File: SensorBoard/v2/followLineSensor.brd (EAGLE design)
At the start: 102.5 x 34.3 mm, 24 parts

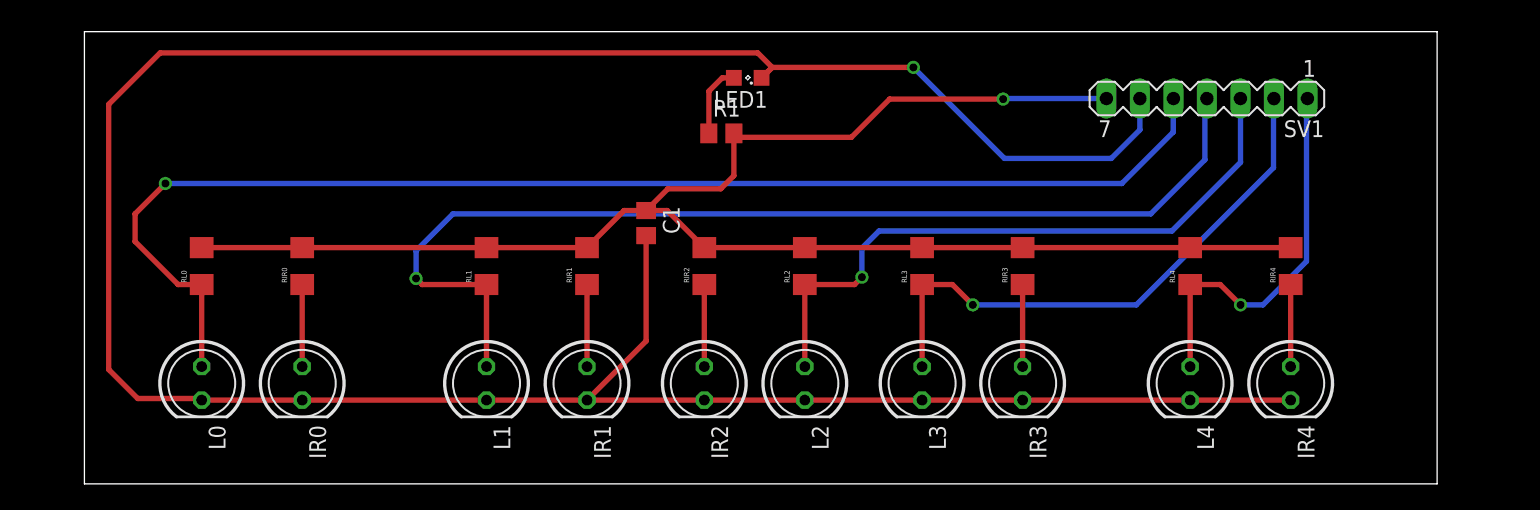
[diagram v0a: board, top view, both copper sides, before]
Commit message: Another better versions of the boards done
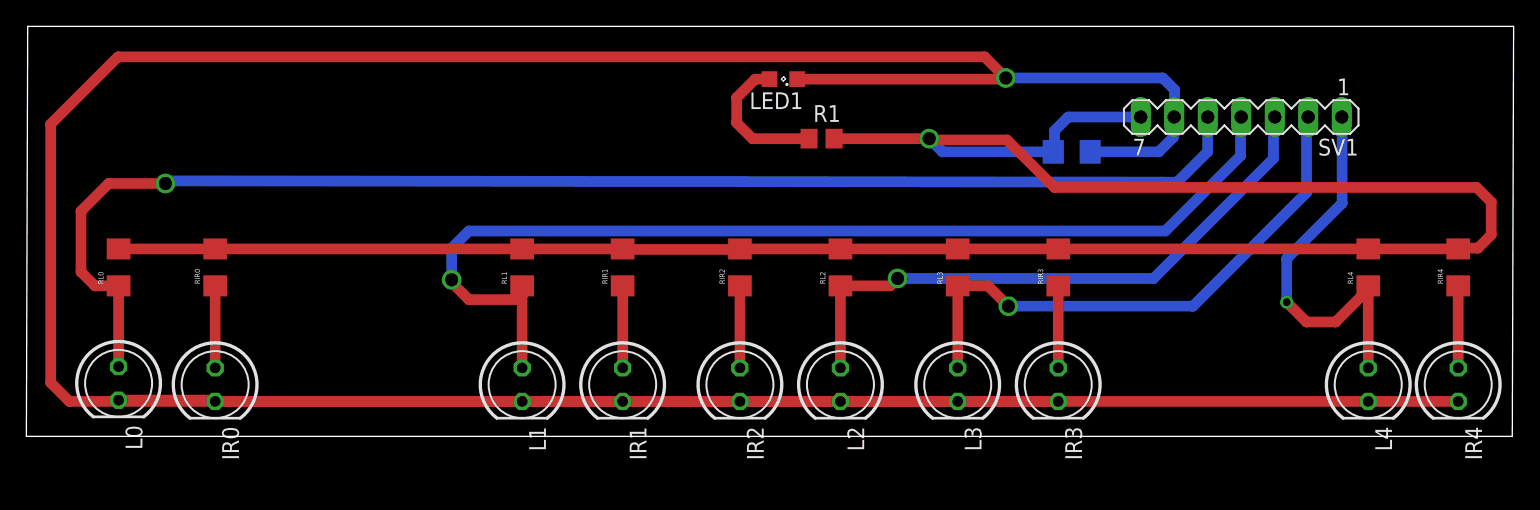
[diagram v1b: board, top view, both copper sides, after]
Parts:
- removed C1: 100nF, rcl:C0805
- added C2: 1uF, rcl:C1206
- moved L4 13.5 mm to (94.8, 44.4)
- moved RL4 13.5 mm to (94.8, 53.2)
- moved IR4 12.7 mm to (101.6, 44.4)
- moved RIR4 12.7 mm to (101.6, 53.2)
- moved R1 7.61 mm to (53.3, 63.0)
- moved IR0 6.60 mm to (7.37, 44.4)
- moved RIR0 6.60 mm to (7.37, 53.2)
- moved RL0 6.30 mm to (0.05, 53.2)
- moved L0 6.30 mm to (0.05, 44.5)
- moved SV1 2.95 mm to (85.2, 64.6)
- moved IR3 2.70 mm to (71.3, 44.4)
- moved L2 2.70 mm to (54.8, 44.4)
- moved RIR3 2.70 mm to (71.3, 53.2)
- moved RL2 2.70 mm to (54.8, 53.2)
- moved L1 2.70 mm to (30.6, 44.4)
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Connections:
- net GND: now also C2.2; no longer C1.2
- net VBAT: now also C2.1; no longer C1.1
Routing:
- net GND: track 213.6 -> 312.8 mm
- net VBAT: track 125.4 -> 177.3 mm
- net N$2: track 5.51 -> 11.0 mm
- net A0: track 98.5 -> 104.0 mm
- net A2: track 49.2 -> 46.4 mm
- net A1: track 81.2 -> 80.5 mm
- net A4: track 29.4 -> 30.1 mm
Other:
- board size 102.5 x 34.3 mm -> 112.7 x 31.1 mm
